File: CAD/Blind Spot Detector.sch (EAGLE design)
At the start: 2 parts, among them IC1 TINY13V-10PU

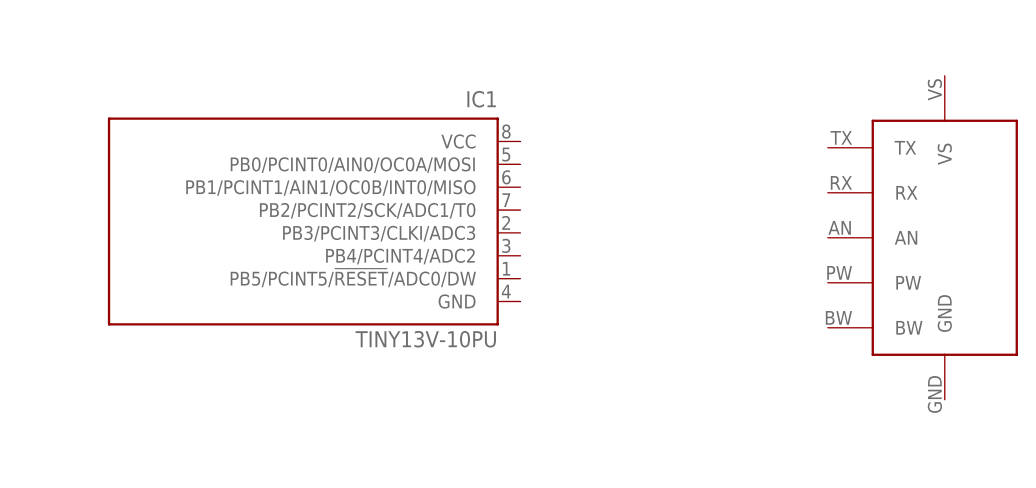
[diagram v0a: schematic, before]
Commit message: Readjusted Grid
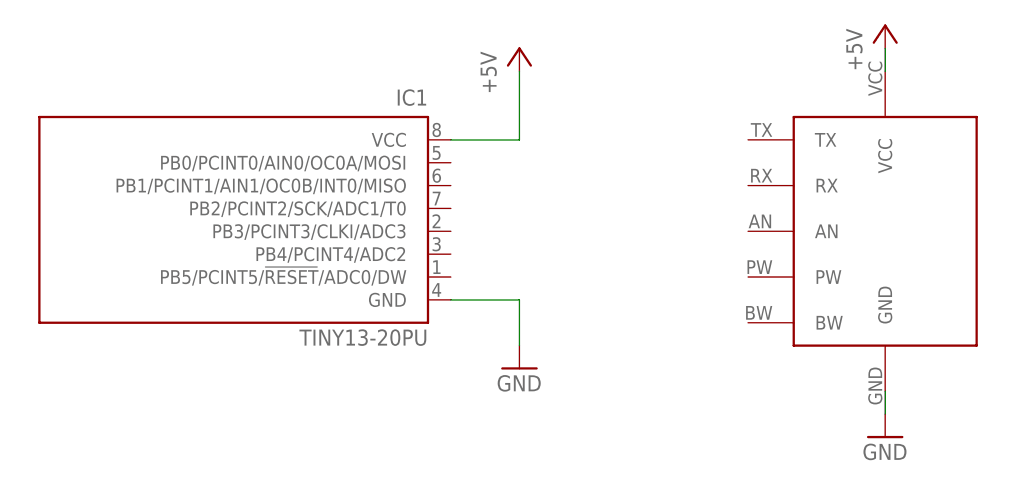
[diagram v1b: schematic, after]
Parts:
- IC1: value TINY13V-10PU -> TINY13-20PU; device atmel:TINY13V-10PU -> atmel:TINY13-20PU
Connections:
- new net +5V: IC1.VCC, U$1.VCC
- new net GND: IC1.GND, U$1.GND
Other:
- moved on the sheet: IC1
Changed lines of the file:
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@@
 </classes>
 <parts>
+<part name="IC1" library="atmel" deviceset="TINY13" device="PU" technology="-20"/>
 <part name="U$1" library="Ultrasonic_sensor" deviceset="ULTRASONIC_SENSOR" device=""/>
-<part name="IC1" library="atmel" deviceset="TINY13" device="PU" technology="V-10"/>
+<part name="P+1" library="supply1" deviceset="+5V" device=""/>
+<part name="P+2" library="supply1" deviceset="+5V" device=""/>
+<part name="GND1" library="supply1" deviceset="GND" device=""/>
+<part name="GND2" library="supply1" deviceset="GND" device=""/>
 </parts>
 <sheets>
@@
 </plain>
 <instances>
-<instance part="U$1" gate="G$1" x="125" y="42"/>
-<instance part="IC1" gate="G$1" x="58.54" y="43" rot="MR0"/>
+<instance part="IC1" gate="G$1" x="50.8" y="43.18" rot="MR0"/>
+<instance part="U$1" gate="G$1" x="116.84" y="40.64"/>
+<instance part="P+1" gate="1" x="78.74" y="66.04"/>
+<instance part="P+2" gate="1" x="119.38" y="68.58"/>
+<instance part="GND1" gate="1" x="119.38" y="22.86"/>
+<instance part="GND2" gate="1" x="78.74" y="30.48"/>
 </instances>
 <busses>
 </busses>
 <nets>
+<net name="GND" class="0">
+<segment>
+<pinref part="IC1" gate="G$1" pin="GND"/>
+<pinref part="GND2" gate="1" pin="GND"/>
+<wire x1="71.12" y1="38.1" x2="78.74" y2="38.1" width="0.1524" layer="91"/>
+<wire x1="78.74" y1="38.1" x2="78.74" y2="33.02" width="0.1524" layer="91"/>
+</segment>
+<segment>
+<pinref part="U$1" gate="G$1" pin="GND"/>
+<pinref part="GND1" gate="1" pin="GND"/>
+<wire x1="119.38" y1="27.94" x2="119.38" y2="25.4" width="0.1524" layer="91"/>
+</segment>
+</net>
+<net name="+5V" class="0">
+<segment>
+<pinref part="IC1" gate="G$1" pin="VCC"/>
+<wire x1="71.12" y1="55.88" x2="78.74" y2="55.88" width="0.1524" layer="91"/>
+<pinref part="P+1" gate="1" pin="+5V"/>
+<wire x1="78.74" y1="55.88" x2="78.74" y2="63.5" width="0.1524" layer="91"/>
+</segment>
+<segment>
+<pinref part="U$1" gate="G$1" pin="VCC"/>
+<pinref part="P+2" gate="1" pin="+5V"/>
+<wire x1="119.38" y1="63.5" x2="119.38" y2="66.04" width="0.1524" layer="91"/>
+</segment>
+</net>
 </nets>
 </sheet>
